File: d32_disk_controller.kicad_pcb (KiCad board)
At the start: 2 copper layers, 107.5 x 80.3 mm, 25 parts, among them J1 Clock_Test, J2 IDC_Floppy, J3 EDGE, U1 27C64, U2 WD2797, U3 74HCT174, U4 74HCT139, U5 74HCT00, U6 74HCT04, U7 74LS07, U8 74HCT74, U9 74HCT04, Y1 4MHz

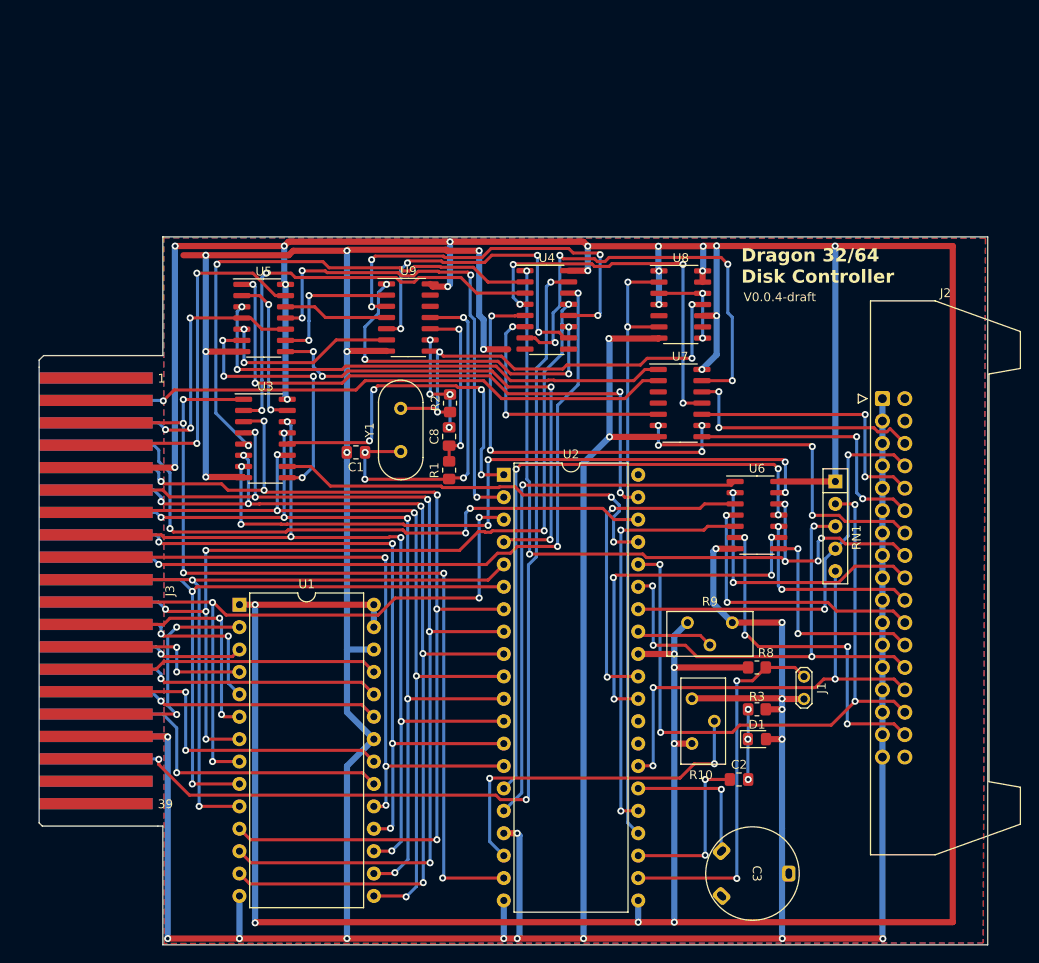
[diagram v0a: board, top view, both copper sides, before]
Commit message: prepare for cpld
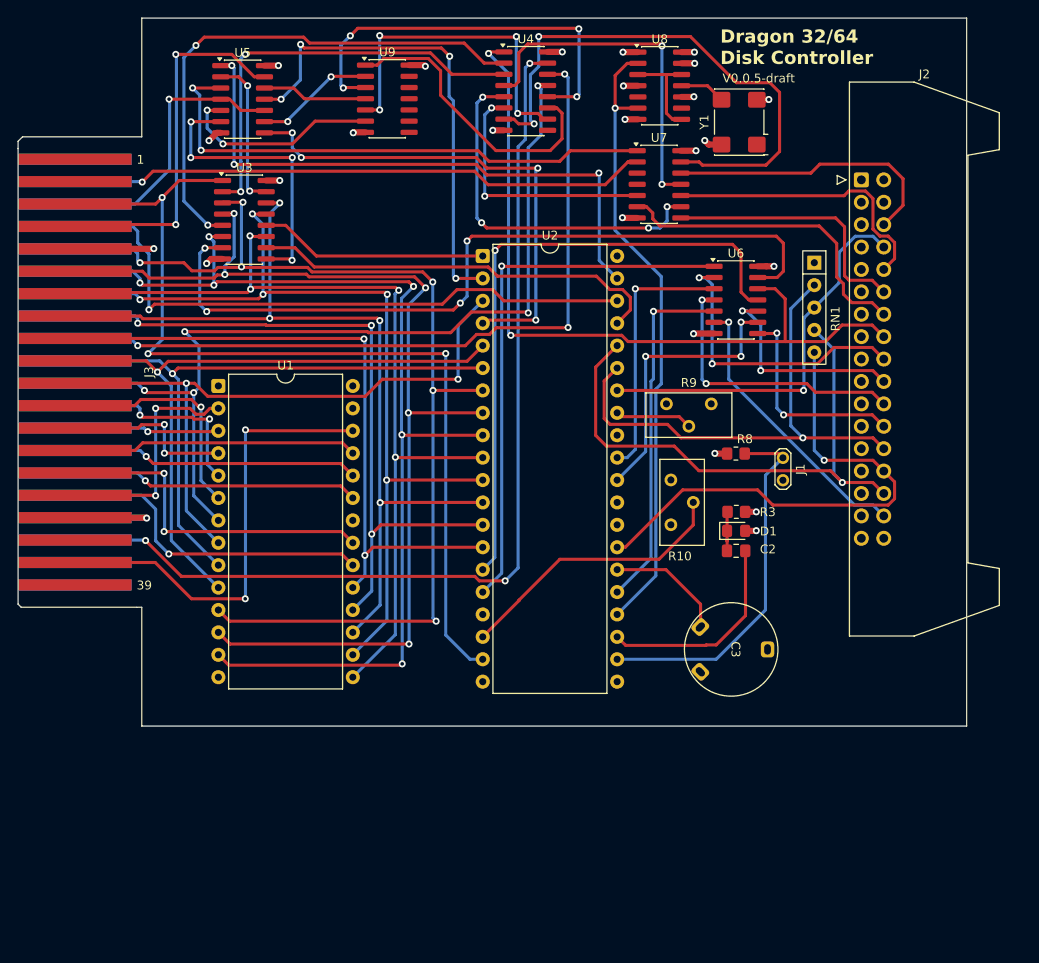
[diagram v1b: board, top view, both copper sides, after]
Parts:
- removed C1: 22pF, Capacitor_SMD:C_0805_2012Metric_Pad1.18x1.45mm_HandSolder
- removed C8: 10nF, Capacitor_SMD:C_0805_2012Metric_Pad1.18x1.45mm_HandSolder
- removed R1, R2: 1K, Resistor_SMD:R_0805_2012Metric_Pad1.20x1.40mm_HandSolder
- Y1: footprint Crystal:Crystal_HC18-U_Vertical -> Oscillator:Oscillator_SMD_Abracon_ASV-4Pin_7.0x5.1mm
- moved Y1 53.5 mm to (129.6, 30.6)
- moved C2 25.9 mm to (129.2, 79.2), turned to 180 degrees
- moved C3 25.5 mm to (128.7, 90.4)
- moved J1 24.9 mm to (134.5, 68.7)
- moved R9 24.9 mm to (126.4, 62.6)
- moved U3 24.9 mm to (73.5, 41.7)
- moved J2 24.9 mm to (143.4, 37.2)
- moved J3 24.9 mm to (63.1, 59.0)
- moved U4 24.9 mm to (105.4, 27.1)
- moved U5 24.9 mm to (73.3, 28.0)
- moved U7 24.9 mm to (120.5, 37.7)
- moved U8 24.9 mm to (120.5, 26.5)
- moved U9 24.9 mm to (89.7, 28.0)
- moved R10 24.9 mm to (121.8, 71.2)
- moved U1 24.9 mm to (70.5, 60.5)
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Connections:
- J3 pad 37: unconnected-(J3-Pin_37-Pad37) -> A13
- RN1 pad 2: ~{WPRT} -> ~{IP}
- RN1 pad 3: ~{IP} -> ~{TR00}
- RN1 pad 4: ~{TR00} -> ~{WPRT}
- U1 pad 26: GND -> A13
- U9 pad 10: Net-(C8-Pad1) -> unconnected-(U9-Pad10)
- U9 pad 11: Net-(C1-Pad1) -> unconnected-(U9-Pad11)
- U9 pad 8: /raw_clock -> unconnected-(U9-Pad8)
- U9 pad 9: Net-(C8-Pad2) -> unconnected-(U9-Pad9)
- Y1 pad 1: Net-(C1-Pad1) -> unconnected-(Y1-EN-Pad1)
- Y1 pad 2: /raw_clock -> GND
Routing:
- net GND: track 524.7 -> 32.1 mm, vias 25 -> 11
- net +5V: track 473.7 -> 30.4 mm, vias 25 -> 14
- net A13: track 0.00 -> 52.4 mm, vias 0 -> 2
- net /raw_clock: track 51.1 -> 5.19 mm, vias 4 -> 0
- net Net-(C1-Pad1): track 40.8 -> 0.00 mm, vias 4 -> 0
- net Net-(C8-Pad1): track 19.6 -> 0.00 mm, vias 2 -> 0
- net ENP: track 40.5 -> 26.0 mm, vias 4 -> 0
- net Net-(C8-Pad2): track 12.3 -> 0.00 mm, vias 4 -> 0
- net Net-(U4A-O3): track 50.7 -> 62.7 mm, vias 4 -> 2
- net ~{WPRT}: track 75.8 -> 65.2 mm, vias 4 -> 1
- net Net-(U3-Q2): track 80.2 -> 89.1 mm, vias 6 -> 4
- net Net-(U2-RPW): track 40.4 -> 31.7 mm, vias 2 -> 0
- net ~{SSO}: track 40.2 -> 32.1 mm, vias 4 -> 1
- net WG: track 39.7 -> 32.0 mm, vias 4 -> 3
- net WD: track 37.1 -> 29.6 mm, vias 2 -> 1
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- added copper zone on In2.Cu, net +5V
- added copper zone on In1.Cu, net GND
- removed copper zone on B.Cu, net GND
- removed copper zone on F.Cu, net GND
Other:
- copper layers 2 -> 4
- board text added: "V0.0.5-draft"
- board text removed: "V0.0.4-draft"
